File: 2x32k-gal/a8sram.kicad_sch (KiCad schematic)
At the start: 17 parts, among them J1 D, U1 GAL16V8, U5 KM62256CLP, U6 KM62256CLP

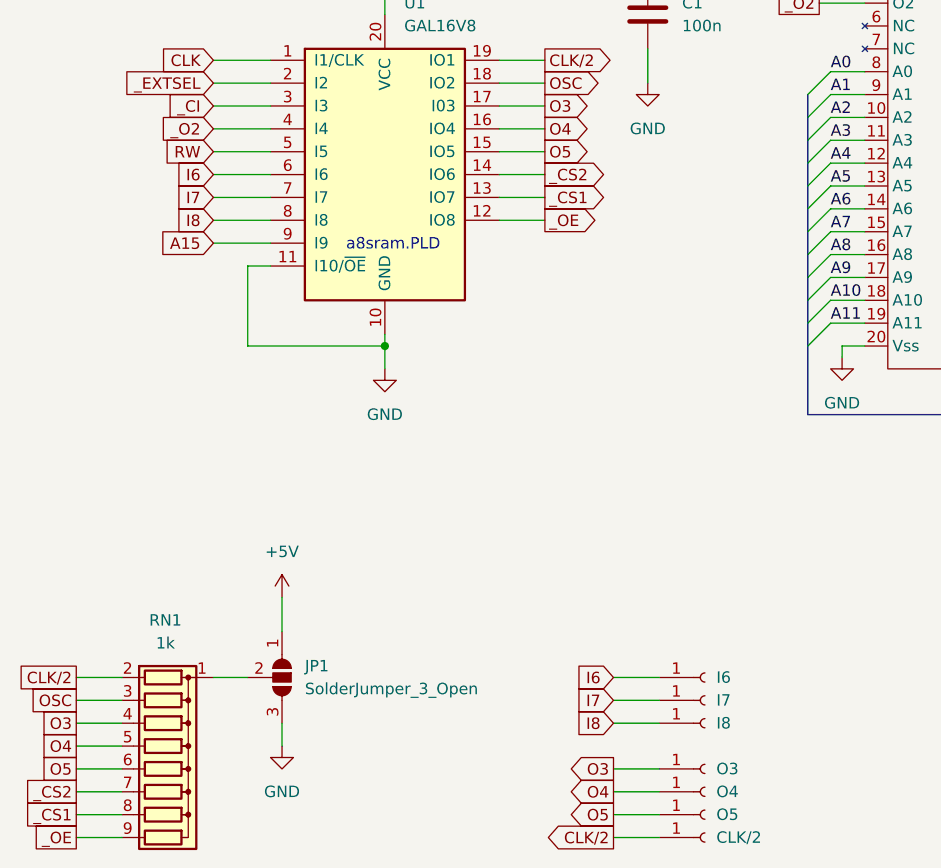
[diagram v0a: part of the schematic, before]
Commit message: Cleanup.
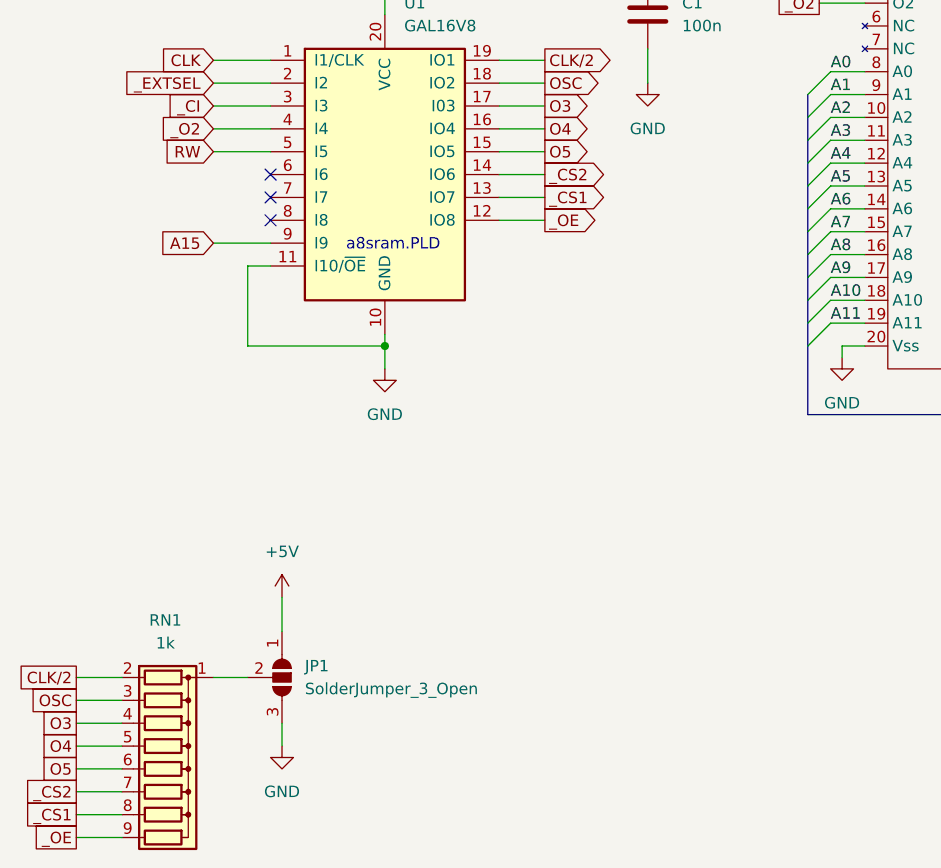
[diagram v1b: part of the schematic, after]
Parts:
- removed CLK/2, I6, I7, I8, O3, O4, O5: ~, Connector_PinHeader_1.00mm:PinHeader_1x01_P1.00mm_Vertical, symbol Connector:Conn_01x01_Socket
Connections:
- net I6: no longer names the net of U1.6 (I6)
- net I7: no longer names the net of U1.7 (I7)
- net I8: no longer names the net of U1.8 (I8)
- no-connect marks 13 -> 16
